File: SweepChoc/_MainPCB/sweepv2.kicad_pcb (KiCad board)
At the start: 2 copper layers, 216.9 x 86.9 mm, 59 parts, among them J1 AudioJack4dpb, J2 AudioJack4dpb, SW1 SW_Push, SW10 SW_Push, SW11 SW_Push, SW11_r1 SW_Push, SW12 SW_Push, SW12_r1 SW_Push, SW13_r1 SW_Push, SW14 SW_Push, SW15 SW_Push, SW15_r1 SW_Push, SW16 SW_Push, SW16_r1 SW_Push, SW17 SW_Push, SW17_r1 SW_Push, SW18 SW_Push, SW18_r1 SW_Push, SW2 SW_Push, SW20 SW_Push, SW21 SW_Push, SW2_r1 SW_Push, SW3 SW_Push, SW3_r1 SW_Push, SW4 SW_Push, SW4_r1 SW_Push, SW5 SW_Push, SW5_r1 SW_Push, SW6 SW_Push, SW6_r1 SW_Push, SW7 SW_Push, SW7_r1 SW_Push, SW8 SW_Push, SW8_r1 SW_Push, SW9 SW_Push, SW9_r1 SW_Push, U1 ProMicro-kbd, U2 ProMicro-kbd

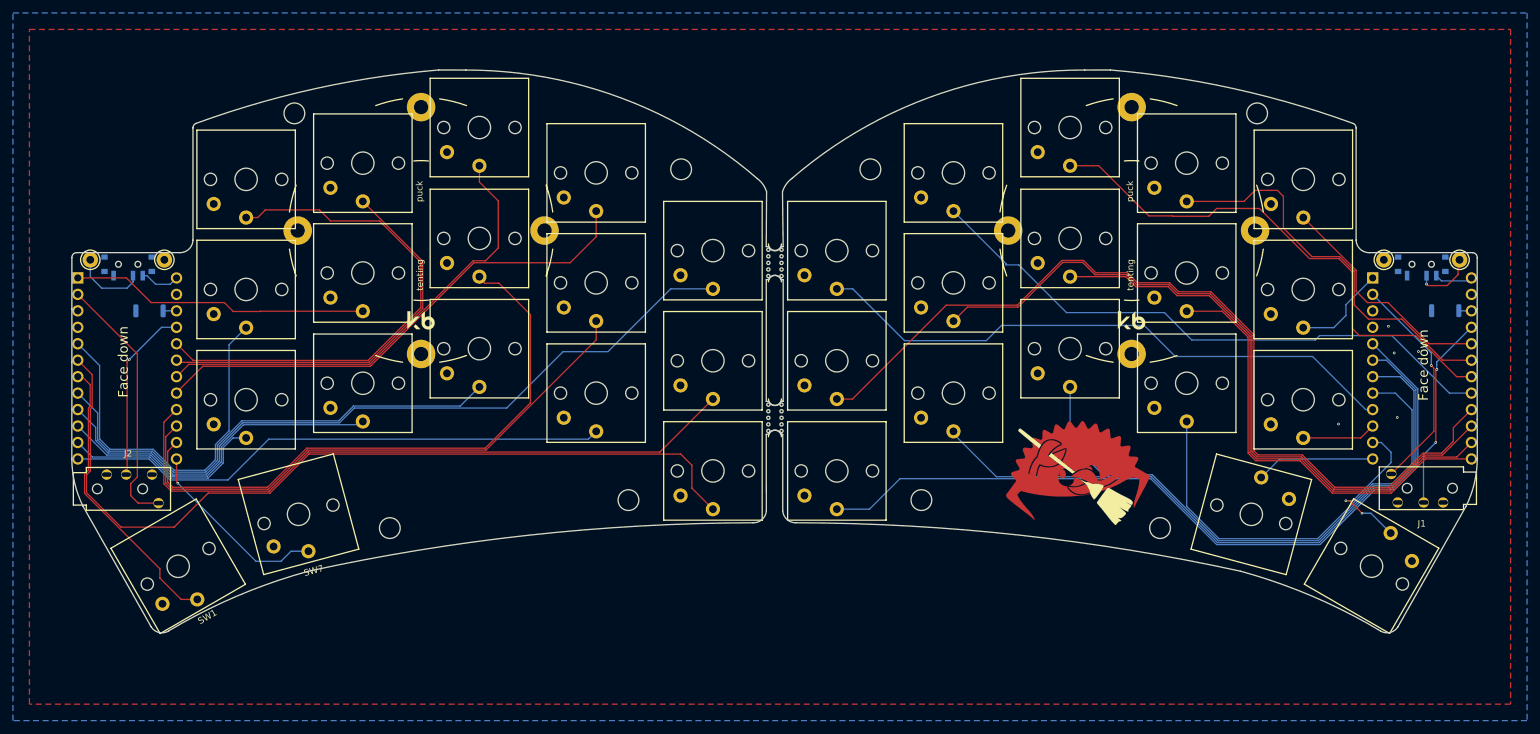
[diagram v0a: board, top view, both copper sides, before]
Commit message: re-worked choc version
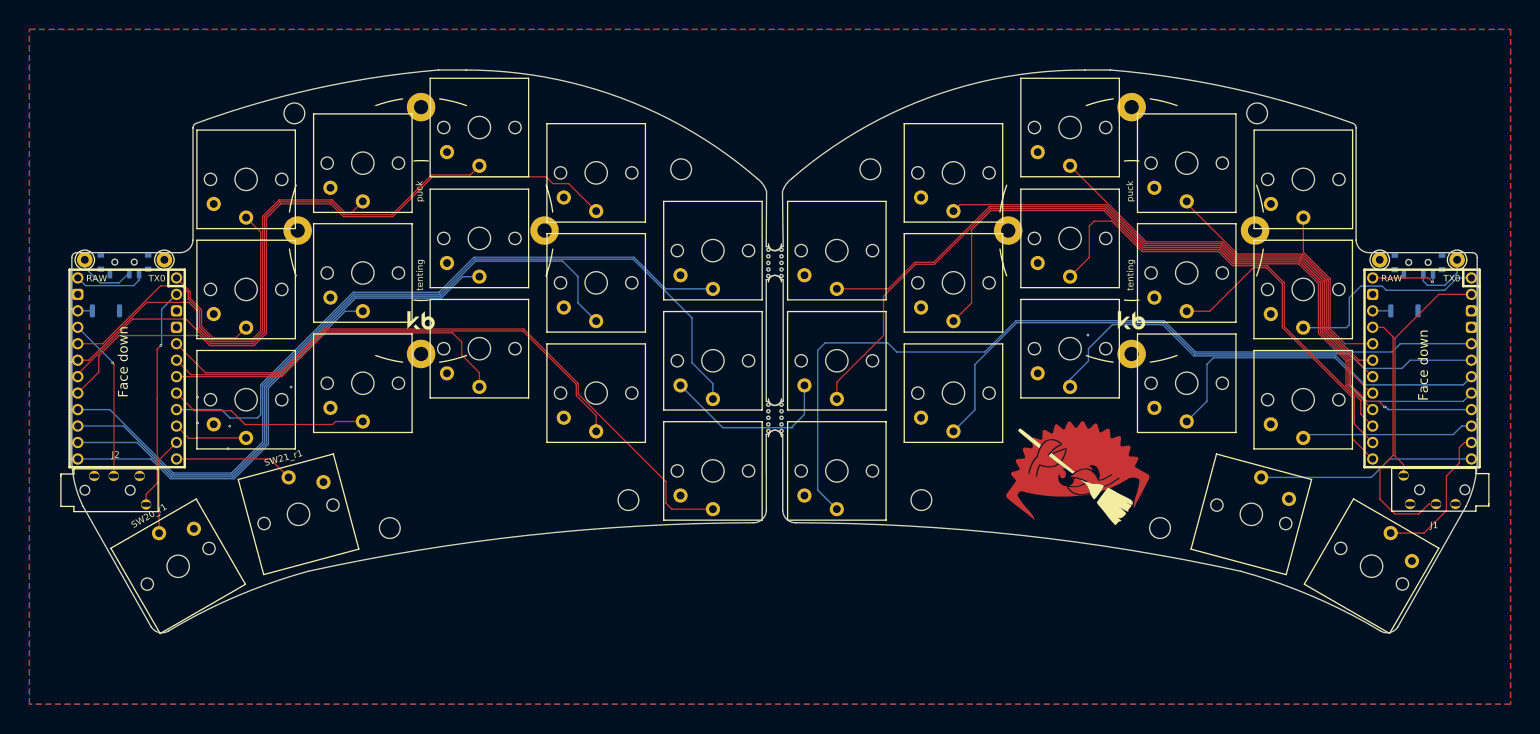
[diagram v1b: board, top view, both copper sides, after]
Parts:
- RSW1, RSW2: value SW_Push -> Reset Button
- U1, U2: moved to B.Cu
- moved Bat+r1 212.2 mm to (23.8, 50.8), turned to 180 degrees
- moved Bat+1 210.9 mm to (235.6, 50.8), turned to 180 degrees
- moved SW_POWERR1 200.2 mm to (29.9, 51.5)
- moved SW_POWER1 199.1 mm to (229.6, 51.5)
- moved RSW2 6.72 mm to (27.1, 58.7), turned to 180 degrees
- moved RSW1 6.29 mm to (227.5, 58.7), turned to 180 degrees
- moved J2 1.93 mm to (20.1, 84.2)
- moved J1 1.93 mm to (240.5, 88.5)
- moved BatGND1 0.64 mm to (223.6, 50.8)
- turned SW20_r1 to 30 degrees
- turned SW21_r1 to 15 degrees
- renumbered SW9_r1 to SW10_r1, SW13_r1 to SW14_r1, SW18_r1 to SW15_r1, SW15_r1 to SW16_r1, SW16_r1 to SW17_r1, SW17_r1 to SW18_r1, SW1 to SW20_r1, SW7 to SW21_r1, SW7_r1 to SW8_r1, SW8_r1 to SW9_r1, mouse-bite-2mm-slot to mouse-bite-2mm-slot-1, mouse-bite-2mm-slot to mouse-bite-2mm-slot-2
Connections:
- J2 pad R1: vcc -> vcc_r
- SW11_r1 pad 1: Switch10_r -> Switch9_r
- SW12_r1 pad 1: Switch11_r -> Switch10_r
- SW14_r1 pad 1: Switch12_r -> Switch11_r
- SW15_r1 pad 1: Switch17_r -> Switch12_r
- SW16_r1 pad 1: Switch14_r -> Switch13_r
- SW17_r1 pad 1: Switch15_r -> Switch14_r
- SW18_r1 pad 1: Switch16_r -> Switch15_r
- SW20_r1 pad 1: Switch13_r -> Switch16_r
- SW21_r1 pad 1: Switch9_r -> Switch17_r
- SW_POWERR1 pad 3: raw -> raw_r
- U2 pad 21: vcc -> vcc_r
- U2 pad 24: raw -> raw_r
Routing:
- net Switch17_r: track 84.5 -> 18.5 mm
- net Switch12_r: track 130.9 -> 77.4 mm
- net Switch14_r: track 76.3 -> 31.0 mm
- net Switch11_r: track 59.0 -> 101.8 mm
- net Switch15_r: track 52.3 -> 11.6 mm
- net Switch2_r: track 78.8 -> 110.9 mm
- net Switch6_r: track 103.4 -> 135.2 mm
- net Switch9_r: track 29.8 -> 61.1 mm, vias 1 -> 0
- net Switch1: track 92.4 -> 122.9 mm, vias 0 -> 1
- net Switch10_r: track 46.2 -> 17.3 mm
- net gnd: track 0.00 -> 27.4 mm, vias 5 -> 6
- net vcc_r: track 0.00 -> 25.3 mm, vias 0 -> 1
- net Switch5_r: track 80.0 -> 56.5 mm
- net Switch7_r: track 88.8 -> 108.1 mm
- net Switch13: track 91.4 -> 72.1 mm
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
